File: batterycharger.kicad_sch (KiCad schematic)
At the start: 27 parts, among them J1 Barrel_Jack, U1 LT3652EMSE

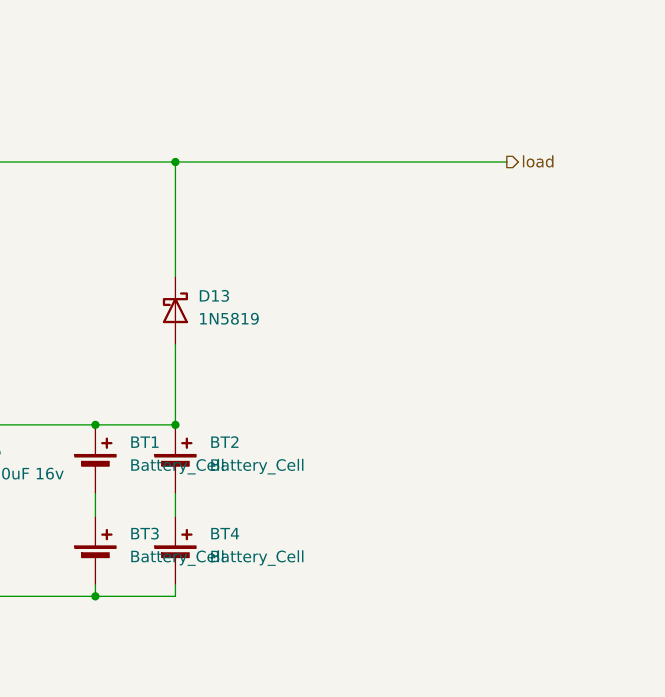
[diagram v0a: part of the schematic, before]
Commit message: Added
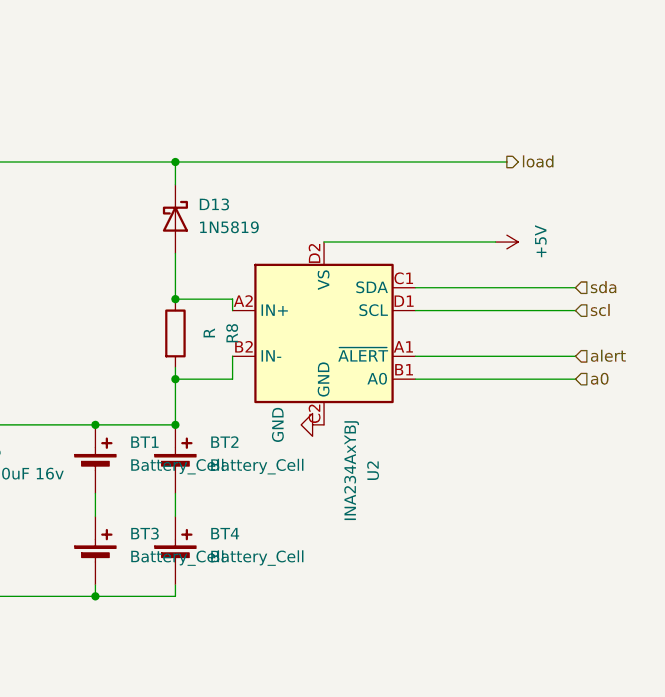
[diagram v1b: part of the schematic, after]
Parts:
- added R8: R, Resistor_THT:R_Axial_DIN0204_L3.6mm_D1.6mm_P5.08mm_Horizontal, symbol Device:R
- added U2: INA234AxYBJ, Package_BGA:Texas_DSBGA-8_0.705x1.468mm_Layout2x4_P0.4mm, symbol Analog_ADC:INA234AxYBJ
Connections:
- net GND: now also U2.C2 (GND)
- net at BT1.1 (+), BT2.1 (+), C2.1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: now also R8.2, U2.B2 (IN-); no longer D13.2 (A)
- new net: D13.2 (A), R8.1, U2.A2 (IN+)
- new net +5V: U2.D2 (VS)
- new net a0: U2.B1 (A0)
- new net alert: U2.A1 (~{ALERT})
- new net scl: U2.D1 (SCL)
- new net sda: U2.C1 (SDA)
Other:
- moved on the sheet: D13
